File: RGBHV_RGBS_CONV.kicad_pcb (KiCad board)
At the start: 2 copper layers, 100 x 100 mm, 40 parts, among them J1 DIGITAL RGB, J11 RGBHV_1, J15 RGBS_OUT, J16 RGBS_OUT, J17 +5V IN, J18 +5V OUT, J2 VGA DB15, J3 ANALOG RGB DA15, J4 X1, J5 DIGITAL_RGBHV_1, J6 ANALOG RGB, J7 DIGITAL_RGBHV_2, J8 ANALOG RGB DA15 EDGE, J9 RGBHV_1, U2 4070/74HC86

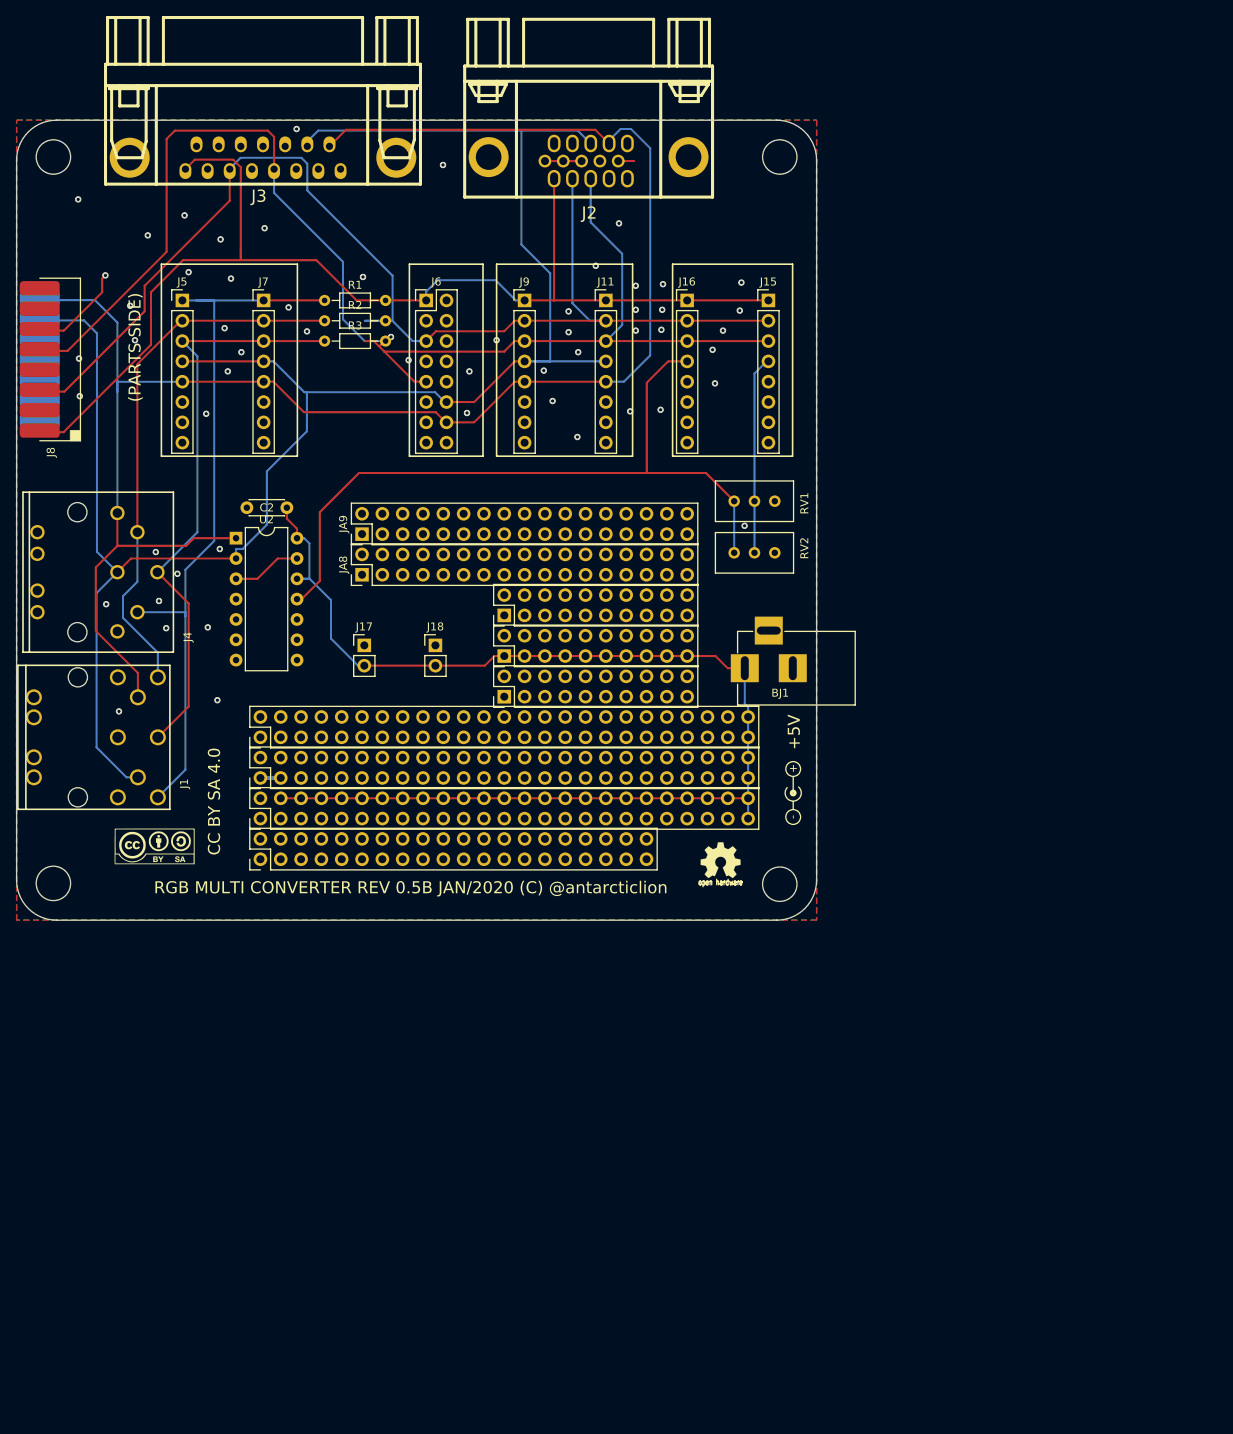
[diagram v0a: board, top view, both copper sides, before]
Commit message: Rev1.0B
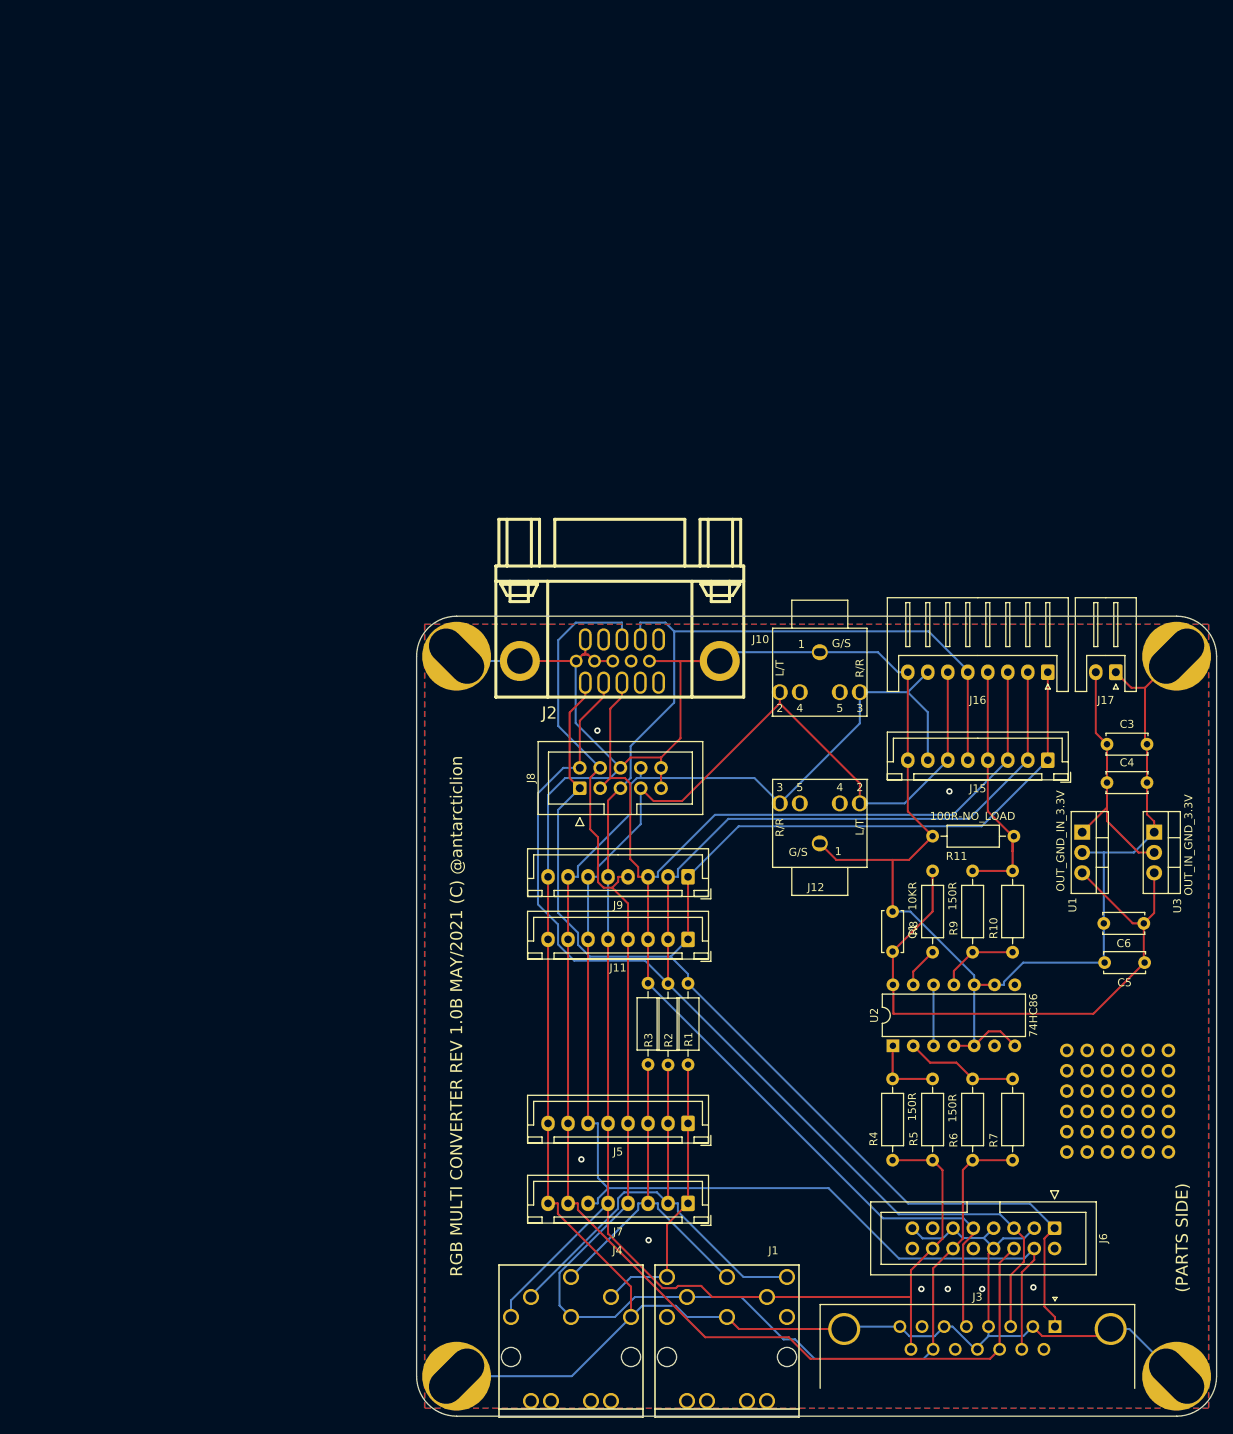
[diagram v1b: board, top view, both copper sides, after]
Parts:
- removed BJ1: BARREL_JACK, Connect:BARREL_JACK
- removed C2: C, Capacitors_ThroughHole:C_Disc_D4.3mm_W1.9mm_P5.00mm
- removed G1, G2: LOGO, w_logo:Logo_silk_CC-BY-SA_10x4.5mm
- removed G3, G4: LOGO, w_logo:Logo_silk_OSHW_6x6mm
- removed J18: +5V OUT, Pin_Headers:Pin_Header_Straight_1x02_Pitch2.54mm
- removed JA1: Pin_Header_Straight_2x20_Pitch2.54mm, Pin_Headers:Pin_Header_Straight_2x20_Pitch2.54mm
- removed JA2, JA3, JA4: Pin_Header_Straight_2x25_Pitch2.54mm, Pin_Headers:Pin_Header_Straight_2x25_Pitch2.54mm
- removed JA5, JA6, JA7: PinHeader_2x10_P2.54mm_Vertical, Connector_PinHeader_2.54mm:PinHeader_2x10_P2.54mm_Vertical
- removed JA8, JA9: PinHeader_2x17_P2.54mm_Vertical, Connector_PinHeader_2.54mm:PinHeader_2x17_P2.54mm_Vertical
- removed REF1, REF2, REF3, REF4: MountingHole_4.3mm_M4, Mounting_Holes:MountingHole_4.3mm_M4
- removed RV1, RV2: R_POT, Potentiometer_THT:Potentiometer_Bourns_3296W_Vertical
- removed SYM1: Symbol_Barrel_Polarity, Symbol:Symbol_Barrel_Polarity
- added C1: 0.1uF, Capacitor_THT:C_Disc_D5.0mm_W2.5mm_P5.00mm, F.Cu at (109.5, 98.9)
- added C3: 10uF, Capacitor_THT:C_Disc_D5.0mm_W2.5mm_P5.00mm, F.Cu at (136.3, 78.0)
- added C4: 0.1uF, Capacitor_THT:C_Disc_D5.0mm_W2.5mm_P5.00mm, F.Cu at (136.3, 82.8)
- added C5: 10uF, Capacitor_THT:C_Disc_D5.0mm_W2.5mm_P5.00mm, F.Cu at (141.0, 105.3)
- added C6: 0.1uF, Capacitor_THT:C_Disc_D5.0mm_W2.5mm_P5.00mm, F.Cu at (140.9, 100.4)
- added H1: M4, MountingHole:MountingHole_4.3mm_M4_Pad, F.Cu at (145.0, 157.0)
- added H2: M4, MountingHole:MountingHole_4.3mm_M4_Pad, F.Cu at (55.0, 67.0)
- added H3: M4, MountingHole:MountingHole_4.3mm_M4_Pad, F.Cu at (55.0, 157.0)
- added H4: M4, MountingHole:MountingHole_4.3mm_M4_Pad, F.Cu at (145.0, 67.0)
- added J10: AUDIO1, ryuk_lib:PJ-3900-04, F.Cu at (100.4, 63.5)
- added J12: AUDIO2, ryuk_lib:PJ-3900-04, F.Cu at (100.4, 93.4)
- added PIN**: Pin_2.54, ryuk_lib:Pin_2.54, F.Cu at (144.0, 126.4)
- added PIN**: Pin_2.54, ryuk_lib:Pin_2.54, F.Cu at (131.3, 126.4)
- added PIN**: Pin_2.54, ryuk_lib:Pin_2.54, F.Cu at (138.9, 129.0)
- added PIN**: Pin_2.54, ryuk_lib:Pin_2.54, F.Cu at (136.4, 129.0)
- added PIN**: Pin_2.54, ryuk_lib:Pin_2.54, F.Cu at (136.4, 121.4)
- added PIN**: Pin_2.54, ryuk_lib:Pin_2.54, F.Cu at (133.8, 121.4)
- added PIN**: Pin_2.54, ryuk_lib:Pin_2.54, F.Cu at (131.3, 121.4)
- added PIN**: Pin_2.54, ryuk_lib:Pin_2.54, F.Cu at (136.4, 123.9)
- added PIN**: Pin_2.54, ryuk_lib:Pin_2.54, F.Cu at (138.9, 123.9)
- added PIN**: Pin_2.54, ryuk_lib:Pin_2.54, F.Cu at (144.0, 123.9)
- added PIN**: Pin_2.54, ryuk_lib:Pin_2.54, F.Cu at (131.3, 123.9)
- added PIN**: Pin_2.54, ryuk_lib:Pin_2.54, F.Cu at (144.0, 129.0)
- added PIN**: Pin_2.54, ryuk_lib:Pin_2.54, F.Cu at (133.8, 123.9)
- added PIN**: Pin_2.54, ryuk_lib:Pin_2.54, F.Cu at (138.9, 121.4)
- added PIN**: Pin_2.54, ryuk_lib:Pin_2.54, F.Cu at (141.4, 121.4)
- added PIN**: Pin_2.54, ryuk_lib:Pin_2.54, F.Cu at (141.4, 123.9)
- added PIN**: Pin_2.54, ryuk_lib:Pin_2.54, F.Cu at (144.0, 121.4)
- added PIN**: Pin_2.54, ryuk_lib:Pin_2.54, F.Cu at (131.3, 116.3)
- added PIN**: Pin_2.54, ryuk_lib:Pin_2.54, F.Cu at (131.3, 118.8)
- added PIN**: Pin_2.54, ryuk_lib:Pin_2.54, F.Cu at (133.8, 118.8)
- added PIN**: Pin_2.54, ryuk_lib:Pin_2.54, F.Cu at (133.8, 116.3)
- added PIN**: Pin_2.54, ryuk_lib:Pin_2.54, F.Cu at (136.4, 118.8)
- added PIN**: Pin_2.54, ryuk_lib:Pin_2.54, F.Cu at (136.4, 126.4)
- added PIN**: Pin_2.54, ryuk_lib:Pin_2.54, F.Cu at (138.9, 118.8)
- added PIN**: Pin_2.54, ryuk_lib:Pin_2.54, F.Cu at (141.4, 118.8)
- added PIN**: Pin_2.54, ryuk_lib:Pin_2.54, F.Cu at (144.0, 118.8)
- added PIN**: Pin_2.54, ryuk_lib:Pin_2.54, F.Cu at (136.4, 116.3)
- added PIN**: Pin_2.54, ryuk_lib:Pin_2.54, F.Cu at (138.9, 116.3)
- added PIN**: Pin_2.54, ryuk_lib:Pin_2.54, F.Cu at (141.4, 116.3)
- added PIN**: Pin_2.54, ryuk_lib:Pin_2.54, F.Cu at (144.0, 116.3)
- added PIN**: Pin_2.54, ryuk_lib:Pin_2.54, F.Cu at (131.3, 129.0)
- added PIN**: Pin_2.54, ryuk_lib:Pin_2.54, F.Cu at (141.4, 129.0)
- added PIN**: Pin_2.54, ryuk_lib:Pin_2.54, F.Cu at (133.8, 129.0)
- added PIN**: Pin_2.54, ryuk_lib:Pin_2.54, F.Cu at (141.4, 126.4)
- added PIN**: Pin_2.54, ryuk_lib:Pin_2.54, F.Cu at (133.8, 126.4)
- added PIN**: Pin_2.54, ryuk_lib:Pin_2.54, F.Cu at (138.9, 126.4)
- added R10: 0R-NO_LOAD, Resistor_THT:R_Axial_DIN0207_L6.3mm_D2.5mm_P10.16mm_Horizontal, F.Cu at (124.5, 104.0)
- added R11: 100R-NO_LOAD, Resistor_THT:R_Axial_DIN0207_L6.3mm_D2.5mm_P10.16mm_Horizontal, F.Cu at (114.5, 89.5)
- added R4: 0R-NO_LOAD, Resistor_THT:R_Axial_DIN0207_L6.3mm_D2.5mm_P10.16mm_Horizontal, F.Cu at (109.5, 130.0)
- added R5: 150R, Resistor_THT:R_Axial_DIN0207_L6.3mm_D2.5mm_P10.16mm_Horizontal, F.Cu at (114.5, 130.0)
- added R6: 150R, Resistor_THT:R_Axial_DIN0207_L6.3mm_D2.5mm_P10.16mm_Horizontal, F.Cu at (119.5, 130.0)
- added R7: 0R-NO_LOAD, Resistor_THT:R_Axial_DIN0207_L6.3mm_D2.5mm_P10.16mm_Horizontal, F.Cu at (124.5, 130.0)
- added R8: 10KR, Resistor_THT:R_Axial_DIN0207_L6.3mm_D2.5mm_P10.16mm_Horizontal, F.Cu at (114.5, 104.0)
- added R9: 150R, Resistor_THT:R_Axial_DIN0207_L6.3mm_D2.5mm_P10.16mm_Horizontal, F.Cu at (119.5, 104.0)
- added U1: OUT_GND_IN_3.3V, Package_TO_SOT_THT:TO-220-3_Vertical, F.Cu at (133.2, 89.0)
- added U3: OUT_IN_GND_3.3V, Package_TO_SOT_THT:TO-220-3_Vertical, F.Cu at (142.2, 89.0)
- J1: footprint ryuk_org_lib:DIN 8 PCB -> ryuk_lib:DIN 8 PCB
- J11: value RGBHV_1 -> RGBHV_2; footprint Pin_Headers:Pin_Header_Straight_1x08_Pitch2.54mm -> Connector_JST:JST_XH_B8B-XH-A_1x08_P2.50mm_Vertical
- J15: value RGBS_OUT -> RGBS_OUT1; footprint Pin_Headers:Pin_Header_Straight_1x08_Pitch2.54mm -> Connector_JST:JST_XH_B8B-XH-A_1x08_P2.50mm_Vertical
- J16: value RGBS_OUT -> RGBS_OUT2; footprint Pin_Headers:Pin_Header_Straight_1x08_Pitch2.54mm -> Connector_JST:JST_XH_S8B-XH-A_1x08_P2.50mm_Horizontal
- J17: value +5V IN -> VIN; footprint Pin_Headers:Pin_Header_Straight_1x02_Pitch2.54mm -> Connector_JST:JST_XH_S2B-XH-A_1x02_P2.50mm_Horizontal
- J2: footprint ryuk_org_lib:DB_15F-VGA_L -> ryuk_lib:DB_15F-VGA_L
- J3: footprint w_conn_d-sub:DB_15F -> Connector_Dsub:DSUB-15_Female_Horizontal_P2.77x2.84mm_EdgePinOffset4.94mm_Housed_MountingHolesOffset7.48mm
- J4: footprint ryuk_org_lib:DIN 6 PCB SDS-60J -> ryuk_lib:DIN_6_PCB
- J5, J7, J9: footprint Pin_Headers:Pin_Header_Straight_1x08_Pitch2.54mm -> Connector_JST:JST_XH_B8B-XH-A_1x08_P2.50mm_Vertical
- J6: footprint Pin_Headers:Pin_Header_Straight_2x08_Pitch2.54mm -> Connector_IDC:IDC-Header_2x08_P2.54mm_Vertical
- J8: value ANALOG RGB DA15 EDGE -> SWITCHER; footprint ryuk_lib:D-SUB15_PCB_EDGE -> Connector_IDC:IDC-Header_2x05_P2.54mm_Vertical
- R1, R2, R3: footprint Resistor_THT:R_Axial_DIN0204_L3.6mm_D1.6mm_P7.62mm_Horizontal -> Resistor_THT:R_Axial_DIN0207_L6.3mm_D2.5mm_P10.16mm_Horizontal
- U2: value 4070/74HC86 -> 74HC86
- moved J3 182.4 mm to (129.8, 150.8), turned to 0 degrees
- moved J6 140.1 mm to (129.8, 138.5), turned to 270 degrees
- moved J7 124.7 mm to (83.9, 135.4), turned to 180 degrees
- moved J5 120.7 mm to (83.9, 125.4), turned to 180 degrees
- moved J4 108.7 mm to (69.3, 152.1), turned to 0 degrees
- moved J1 108.6 mm to (88.8, 152.1), turned to 0 degrees
- moved R1 105.8 mm to (83.9, 118.1), turned to 90 degrees
- moved U2 103.8 mm to (109.5, 115.7), turned to 90 degrees
- moved R2 102.4 mm to (81.4, 118.1), turned to 90 degrees
- moved R3 99.1 mm to (78.9, 118.0), turned to 90 degrees
- moved J17 94.0 mm to (137.4, 69.0), turned to 180 degrees
- moved J8 81.0 mm to (70.4, 83.5)
- moved J11 80.5 mm to (83.9, 102.4), turned to 180 degrees
- moved J9 74.9 mm to (83.9, 94.6), turned to 180 degrees
- moved J15 67.2 mm to (128.9, 80.0), turned to 180 degrees
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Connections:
- J11 pad 6: Net-(J11-Pad6) -> AUDIO_L
- J11 pad 7: Net-(J11-Pad7) -> AUDIO_R
- J15 pad 4: CSYNC_RE -> CSYNC
- J15 pad 5: Net-(J15-Pad5) -> VSYNC
- J15 pad 6: Net-(J15-Pad6) -> AUDIO_L
- J15 pad 7: Net-(J15-Pad7) -> AUDIO_R
- J16 pad 5: Net-(J16-Pad5) -> VSYNC
- J16 pad 6: Net-(J16-Pad6) -> AUDIO_L
- J16 pad 7: Net-(J16-Pad7) -> AUDIO_R
- J17 pad 2: +5V -> Net-(C3-Pad1)
- J3 pad 10: Net-(J3-Pad10) -> AUDIO_L
- J3 pad 11: Net-(J3-Pad11) -> AUDIO_R
- J3 pad 12: Net-(J3-Pad12) -> GND
- J3 pad 8: Net-(J3-Pad8) -> GND
- J5 pad 6: Net-(J5-Pad6) -> AUDIO_L
- J5 pad 7: Net-(J5-Pad7) -> AUDIO_R
- J6 pad 15: Net-(J6-Pad15) -> GND
- J6 pad 4: Net-(J6-Pad4) -> AUDIO_L
- J6 pad 6: Net-(J6-Pad6) -> AUDIO_R
- J6 pad 8: Net-(J6-Pad8) -> GND
- J7 pad 6: Net-(J7-Pad6) -> AUDIO_L
- J7 pad 7: Net-(J7-Pad7) -> AUDIO_R
- J8 pad 10: Net-(J8-Pad10) -> GND
- J8 pad 2: GND -> G
- J8 pad 3: G -> B
- J8 pad 4: GND -> HSYNC
- J8 pad 5: B -> VSYNC
- J8 pad 7: Net-(J8-Pad7) -> AUDIO_L
- J8 pad 8: Net-(J8-Pad8) -> AUDIO_R
- J8 pad 9: Net-(J8-Pad9) -> GND
- J9 pad 6: Net-(J9-Pad6) -> AUDIO_L
- J9 pad 7: Net-(J9-Pad7) -> AUDIO_R
- U2 pad 1: VSYNC -> Net-(R4-Pad2)
- U2 pad 10: Net-(U2-Pad10) -> GND
- U2 pad 11: CSYNC -> Net-(R10-Pad1)
- U2 pad 12: +5V -> Net-(U2-Pad12)
- U2 pad 13: Net-(U2-Pad13) -> Net-(R8-Pad1)
- U2 pad 14: +5V -> +3V3
- U2 pad 2: HSYNC -> Net-(R6-Pad2)
- U2 pad 3: Net-(U2-Pad13) -> Net-(U2-Pad12)
- U2 pad 4: Net-(U2-Pad4) -> GND
- U2 pad 5: Net-(U2-Pad5) -> GND
- U2 pad 9: Net-(U2-Pad9) -> GND
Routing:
- net GND: track 21.1 -> 454.1 mm, vias 56 -> 8
- net AUDIO_L: track 0.00 -> 194.9 mm
- net AUDIO_R: track 0.00 -> 191.8 mm
- net +5V: track 153.9 -> 0.00 mm
- net +3V3: track 0.00 -> 76.1 mm
- net CSYNC: track 94.7 -> 33.1 mm
- net DIGITAL_R: track 91.5 -> 35.7 mm
- net R: track 144.9 -> 197.5 mm
- net G: track 150.9 -> 199.5 mm
- net HSYNC: track 235.8 -> 188.6 mm
- net Net-(C3-Pad1): track 0.00 -> 31.1 mm
- net DIGITAL_B: track 73.4 -> 45.3 mm
- net CSYNC_RE: track 24.8 -> 0.00 mm
- net Net-(R6-Pad2): track 0.00 -> 14.1 mm
- net Net-(R10-Pad1): track 0.00 -> 10.0 mm
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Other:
- board text added: "+5_12V"
- board text added: "GND"
- board text added: "RGB MULTI CONVERTER REV 1.0B MAY/2021 (C) @antarcticlion"
- board text removed: "+"
- board text removed: "+5V"
- board text removed: "-"
- board text removed: "ANALOG RGB HV"
- board text removed: "ANALOG RGB S"
- board text removed: "CC BY SA 4.0"
- board text removed: "DIGITAL RGB HV"
- board text removed: "RGB MULTI CONVERTER REV 0.5B JAN/2020 (C) @antarcticlion"
